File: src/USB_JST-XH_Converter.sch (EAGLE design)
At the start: 45 parts, among them SW1 SS-12D00G3, U1 TCKE805NAWSON10B_TOS-REC, U2 TC75S56F

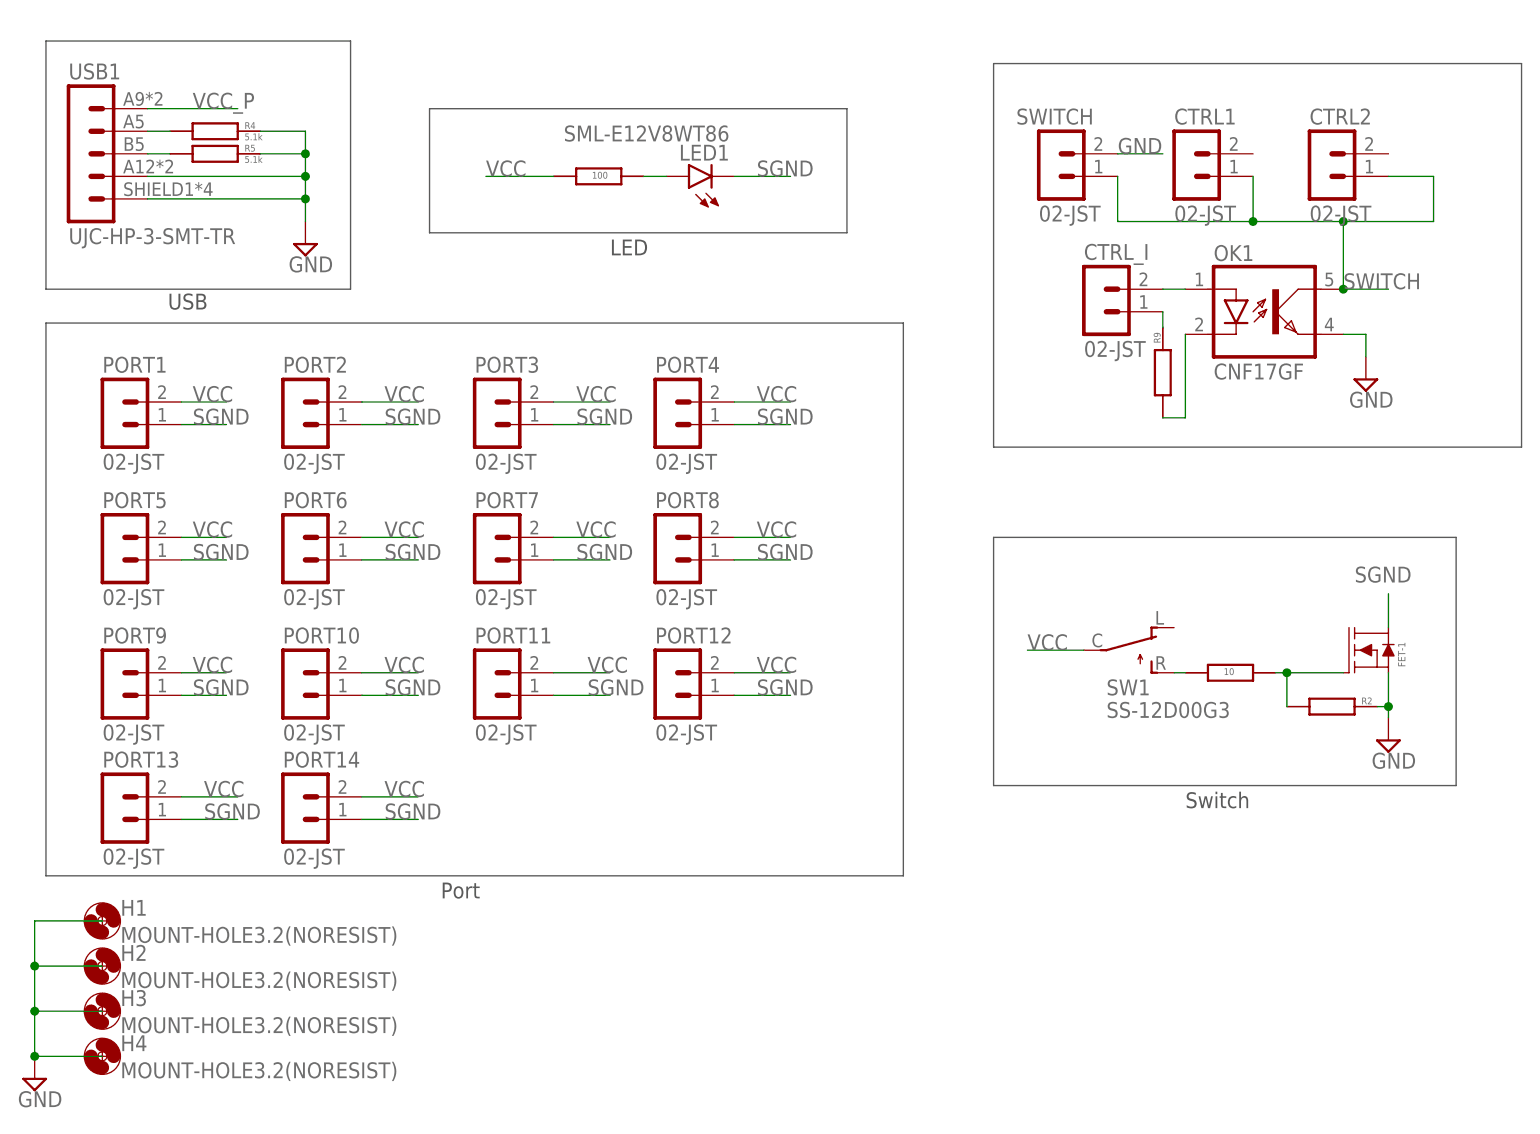
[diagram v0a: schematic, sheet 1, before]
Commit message: 回路図仮完成
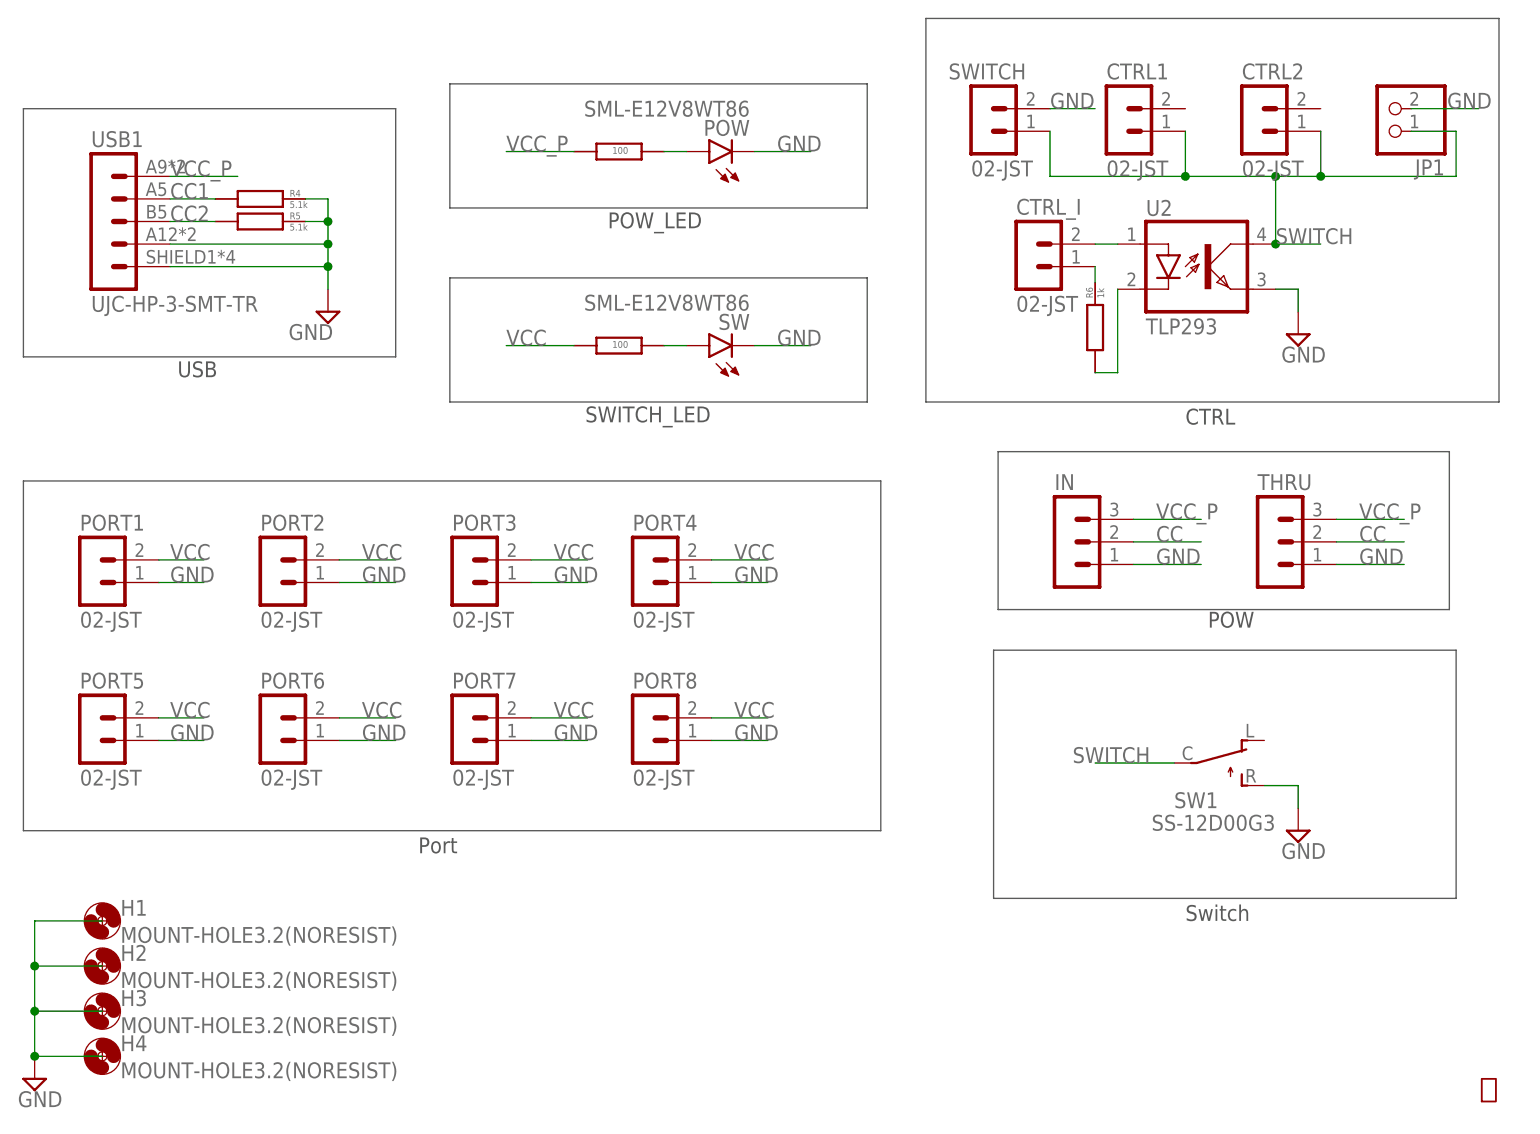
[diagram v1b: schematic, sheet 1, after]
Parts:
- removed FET-1: IRLR6225, OKUDA_libraries:IRLR6225
- removed LED1: SML-E12V8WT86, SML-E12V8WT86:SML-E12V8WT86
- removed OK1: CNF17GF, optocoupler:CNF17GF
- removed PORT10, PORT11, PORT12, PORT13, PORT14, PORT9: 02-JST, con-jst-xh:02-JST
- removed R2, R9: 10k, RG2012:RG2012
- added C4: UWT1E221MNL1GS, UWT1E221MNL1GS:UWT1E221MNL1GS
- added COMP1: MCP6541T-I/LT, MCP6541T-I:MCP6541T-I/LT
- added D3, D4: RB751S40, RB751S40:RB751S40
- added FET1: BSS138, BSS138:BSS138
- added IN, THRU: (no value), con-jst-xh:03-JST
- added JP1: (no value), pinhead:PINHD-1X2
- added POW, SW: SML-E12V8WT86, SML-E12V8WT86:SML-E12V8WT86
- added R12: 10, RG2012:RG2012
- added R13, R16: 10k, RG2012:RG2012
- added R14: 69.8k, RG2012:RG2012
- added R15: 75k, RG2012:RG2012
- added TP1: GF063PB302K, GF063P B104K:GF063PB302K
- added TR1: 2SC3325, 2SC3325:2SC3325
- C3: value GRM21BC72A105KE01 -> GRM1885C1H242JA01D; device GRM21BC72A105KE01(1uF):GRM21BC72A105KE01 -> GRM1885C1H242JA01D:GRM1885C1H242JA01D
- D1: value (none) -> RB751S40; device diode:SCHOTTKY-DIODEF126Z12 -> RB751S40:RB751S40
- D2: value ZZ22 -> PJSD12TS; device diode:ZZ22 -> PJSD12TS:PJSD12TS
- R1: value RG2012Q-100-D-T5 -> RG2012N-101-B-T5; device RG2012Q-100-D-T5:RG2012Q-100-D-T5 -> RG2012N-101-B-T5:RG2012N-101-B-T5
- R10, R7: value (none) -> 10k
- R11: value (none) -> 2.7k
- R6: value (none) -> 1k
- R8: value (none) -> 3k
- U2: value TC75S56F -> TLP293; device TC75S56F:TC75S56F -> TLP293:TLP293
- USB1: device UJC-HP-3-SMT-TR:UJC-HP-3-SMT-TR -> UJC-HP-3-SMT-TRv2:UJC-HP-3-SMT-TR
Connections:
- removed net N$11: R10.RIGHT, R11.RIGHT, U2.3
- removed net SGND: FET-1.D, LED1.C, PORT1.1, PORT10.1, PORT11.1, PORT12.1, PORT13.1, PORT14.1, PORT2.1, PORT3.1, PORT4.1, PORT5.1, PORT6.1, PORT7.1, PORT8.1, PORT9.1
- new net CC: COMP1.IN+, D3.C, D4.C, IN.2, THRU.2
- new net CC1: D3.A, R4.LEFT, USB1.CC1
- new net CC2: D4.A, R5.LEFT, USB1.CC2
- new net ILIM: R14.LEFT, R15.LEFT, U1.ILIM
- new net N$12: COMP1.OUT, R12.RIGHT
- new net N$15: FET1.D, R14.RIGHT
- net GND: now also C3.2, C4.CATHODE, COMP1.VSS, D2.A, FET1.S, IN.1, JP1.2, PORT1.1, PORT2.1, PORT3.1, PORT4.1, PORT5.1, PORT6.1, PORT7.1, PORT8.1, POW.C, R11.RIGHT, R13.RIGHT, R15.RIGHT, SW.C, SW1.R, THRU.1, TR1.E, U2.3; no longer C3.P$2, D2.1, FET-1.S, OK1.EMIT, R11.LEFT, R2.RIGHT, R6.LEFT
- net N$1: now also POW.A, R1.P$1; no longer R1.P$2, SW1.R
- net N$10: now also R6.LEFT, U2.2; no longer OK1.C, R9.LEFT
- net N$2: now also R8.RIGHT, TP1.LEFT, TR1.C, U1.EN/UVLO; no longer FET-1.G, R1.P$1, R2.LEFT
- net N$3: now also SW.A; no longer LED1.A
- net N$4: now also COMP1.IN-, R10.LEFT, R11.LEFT; no longer R4.LEFT, USB1.CC1
- net N$5: now also FET1.G, R12.LEFT, R13.LEFT; no longer R5.LEFT, USB1.CC2
- net N$6: now also R7.LEFT, TP1.RIGHT; no longer R6.RIGHT, U1.ILIM
- net N$7: now also C3.1; no longer C3.P$1
- net N$8: now also U2.1; no longer OK1.A
- net N$9: now also R6.RIGHT; no longer R9.RIGHT
- net SWITCH: now also JP1.1, R16.LEFT, SW1.C, TR1.B, U2.4; no longer OK1.COL, R7.LEFT, R8.RIGHT, U1.EN/UVLO
- net VCC: now also C4.ANODE; no longer PORT10.2, PORT11.2, PORT12.2, PORT13.2, PORT14.2, PORT9.2, SW1.C
- net VCC_P: now also COMP1.VDD, D2.C, IN.3, R1.P$2, R10.RIGHT, R16.RIGHT, THRU.3; no longer D2.2, R10.LEFT
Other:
- note added: "CTRL"
- note added: "Current Supply Capability Discrimination Circuit"
- note added: "POW"
- note added: "POW_LED"
- note added: "SWITCH_LED"
- note added: "eFuse"
- note added: "完"
- note removed: "LED"
- moved on the sheet: C1, C2, CTRL1, CTRL2, CTRL_I, D1, PORT1, PORT2, PORT3, PORT4, PORT5, PORT6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
